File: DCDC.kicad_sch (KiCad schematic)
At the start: 18 parts, among them IC1 AZ1117CH-3.3TRG1

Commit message: コンデンサを追加
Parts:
- removed C10, C7: 10µF, Capacitor_SMD:C_0805_2012Metric_Pad1.18x1.45mm_HandSolder, symbol Device:C
- removed C10, C9: 47u, Capacitor_SMD:C_0805_2012Metric_Pad1.18x1.45mm_HandSolder, symbol Device:C
- removed C3: 0.1μF, Capacitor_SMD:C_0603_1608Metric_Pad1.08x0.95mm_HandSolder, symbol Device:C
- removed C4: 0.01μF, Capacitor_SMD:C_0603_1608Metric_Pad1.08x0.95mm_HandSolder, symbol Device:C
- removed C5, C6, C7, C8: 47u, Capacitor_SMD:C_1210_3225Metric_Pad1.33x2.70mm_HandSolder, symbol Device:C
- removed IC1: AZ1117CH-3.3TRG1, Library:SOT230P700X180-4N, symbol SamacSys_Parts:AZ1117CH-3.3TRG1
- removed L1: CDRH127_LDNP-560MC, Library:INDPM7066X300N, symbol CDRH127_LDNP-560MC:CDRH127_LDNP-560MC
- removed PS1: BP5293-50, Library:TO254P570X1700X1780-3P, symbol BP5293-50:BP5293-50
- removed R1, R2, R3: R, Resistor_SMD:R_0603_1608Metric_Pad0.98x0.95mm_HandSolder, symbol Device:R
- removed U1: ~, Package_SO:SOIC-8-1EP_3.9x4.9mm_P1.27mm_EP2.95x4.9mm_Mask2.71x3.4mm, symbol AP64502:AP64502
- removed VR1: 3362P-1-103LF, Library:3362P_1, symbol 3362P-1-103LF:3362P-1-103LF

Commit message: 電流センサー変更
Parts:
- added C10, C9: 47u, Capacitor_SMD:C_0805_2012Metric_Pad1.18x1.45mm_HandSolder, symbol Device:C
- added C3: 0.1μF, Capacitor_SMD:C_0603_1608Metric_Pad1.08x0.95mm_HandSolder, symbol Device:C
- added C4: 0.01μF, Capacitor_SMD:C_0603_1608Metric_Pad1.08x0.95mm_HandSolder, symbol Device:C
- added C45, C46: 10µF, Capacitor_SMD:C_0805_2012Metric_Pad1.18x1.45mm_HandSolder, symbol Device:C
- added C5, C6, C7, C8: 47u, Capacitor_SMD:C_1210_3225Metric_Pad1.33x2.70mm_HandSolder, symbol Device:C
- added IC11: AZ1117CH-3.3TRG1, Library:SOT230P700X180-4N, symbol SamacSys_Parts:AZ1117CH-3.3TRG1
- added L1: CDRH127_LDNP-560MC, Library:INDPM7066X300N, symbol CDRH127_LDNP-560MC:CDRH127_LDNP-560MC
- added PS2: BP5293-50, Library:TO254P570X1700X1780-3P, symbol BP5293-50:BP5293-50
- added R1 (x2): 100kΩ, Resistor_SMD:R_0603_1608Metric_Pad0.98x0.95mm_HandSolder, symbol Device:R
- added R2, R3: R, Resistor_SMD:R_0603_1608Metric_Pad0.98x0.95mm_HandSolder, symbol Device:R
- added U1: ~, Package_SO:SOIC-8-1EP_3.9x4.9mm_P1.27mm_EP2.95x4.9mm_Mask2.71x3.4mm, symbol AP64502:AP64502
- added VR1: 3362P-1-103LF, Library:3362P_1, symbol 3362P-1-103LF:3362P-1-103LF
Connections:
- new net: C3.2, L1.1, U1.8 (SW)
- new net: R1.1, U1.4 (RT/CLK)
- new net: R1.1, R1.2
- new net: R2.1, VR1.2 (WIPER)
- new net: R2.2, R3.1, U1.5 (FB)
- new net: C4.1, U1.6 (SS)
- new net: C3.1, U1.1 (BST)
- new net +5V: C45.1, IC11.3 (INPUT), PS2.3 (VOUT)
- new net 3.3V: C46.1, IC11.2 (OUTPUT), IC11.4 (VOUT)
- new net GND: C10.2, C4.2, C45.2, C46.2, C5.2, C6.2, C7.2, C8.2, C9.2, IC11.1 (ADJ/GND), PS2.2 (GND), R1.2, R3.2, U1.7 (GND), U1.9 (GND)
- new net VIN: C10.1, C9.1, PS2.1 (VIN), U1.2 (VIN), U1.3 (EN)
- new net VOUT: C5.1, C6.1, C7.1, C8.1, L1.2, VR1.3 (CW)

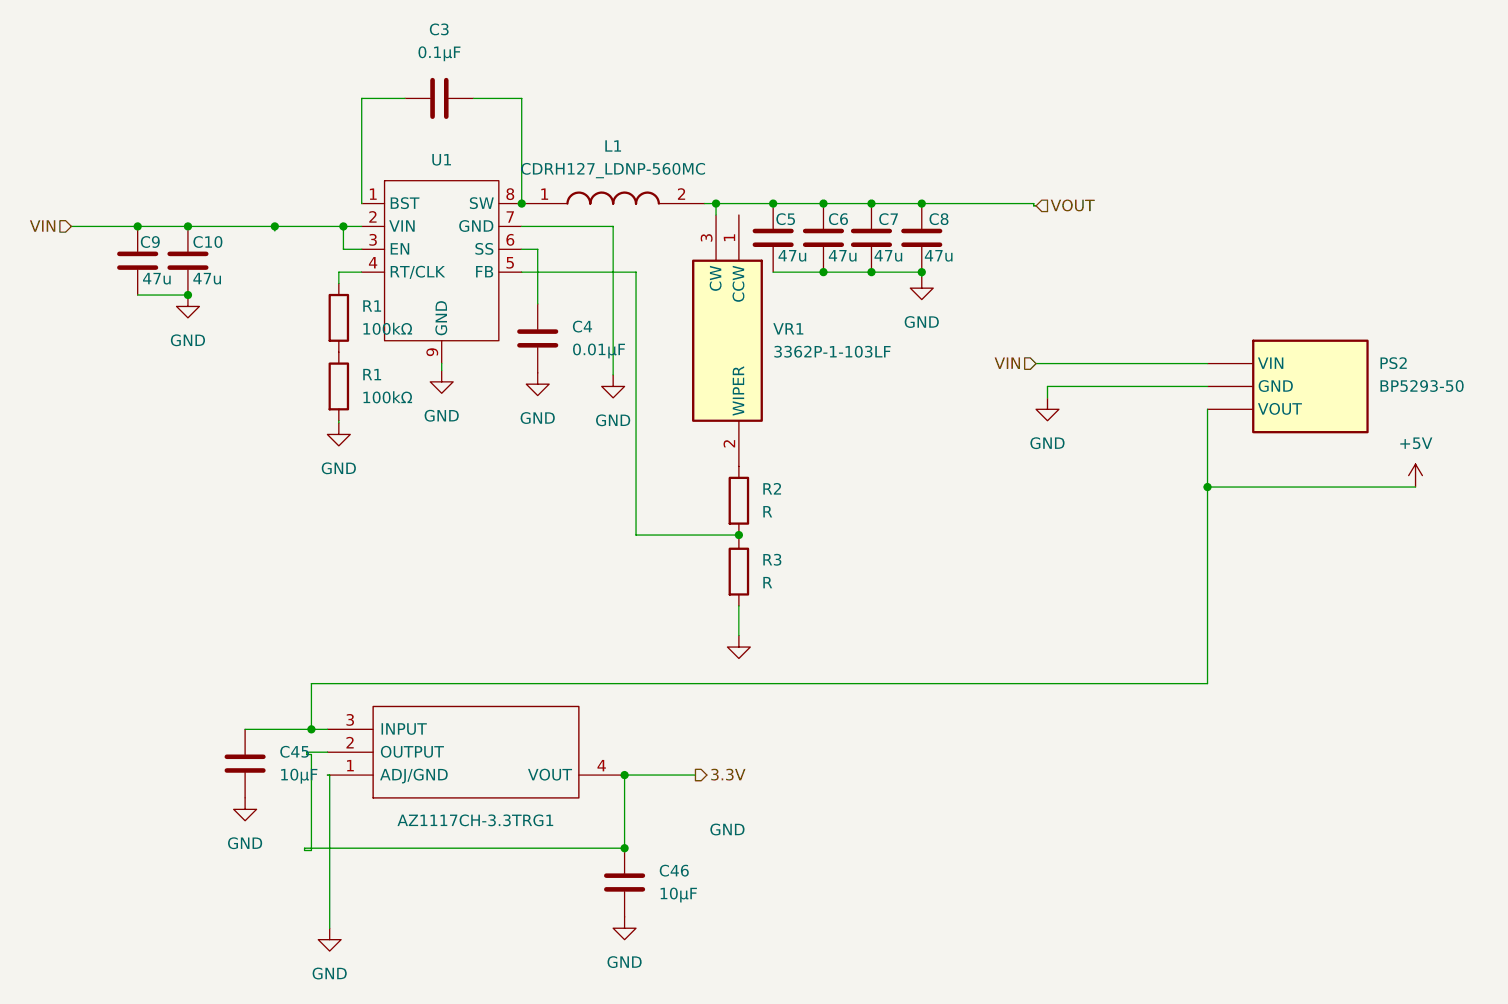
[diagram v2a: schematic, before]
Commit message: ESP32バージョン
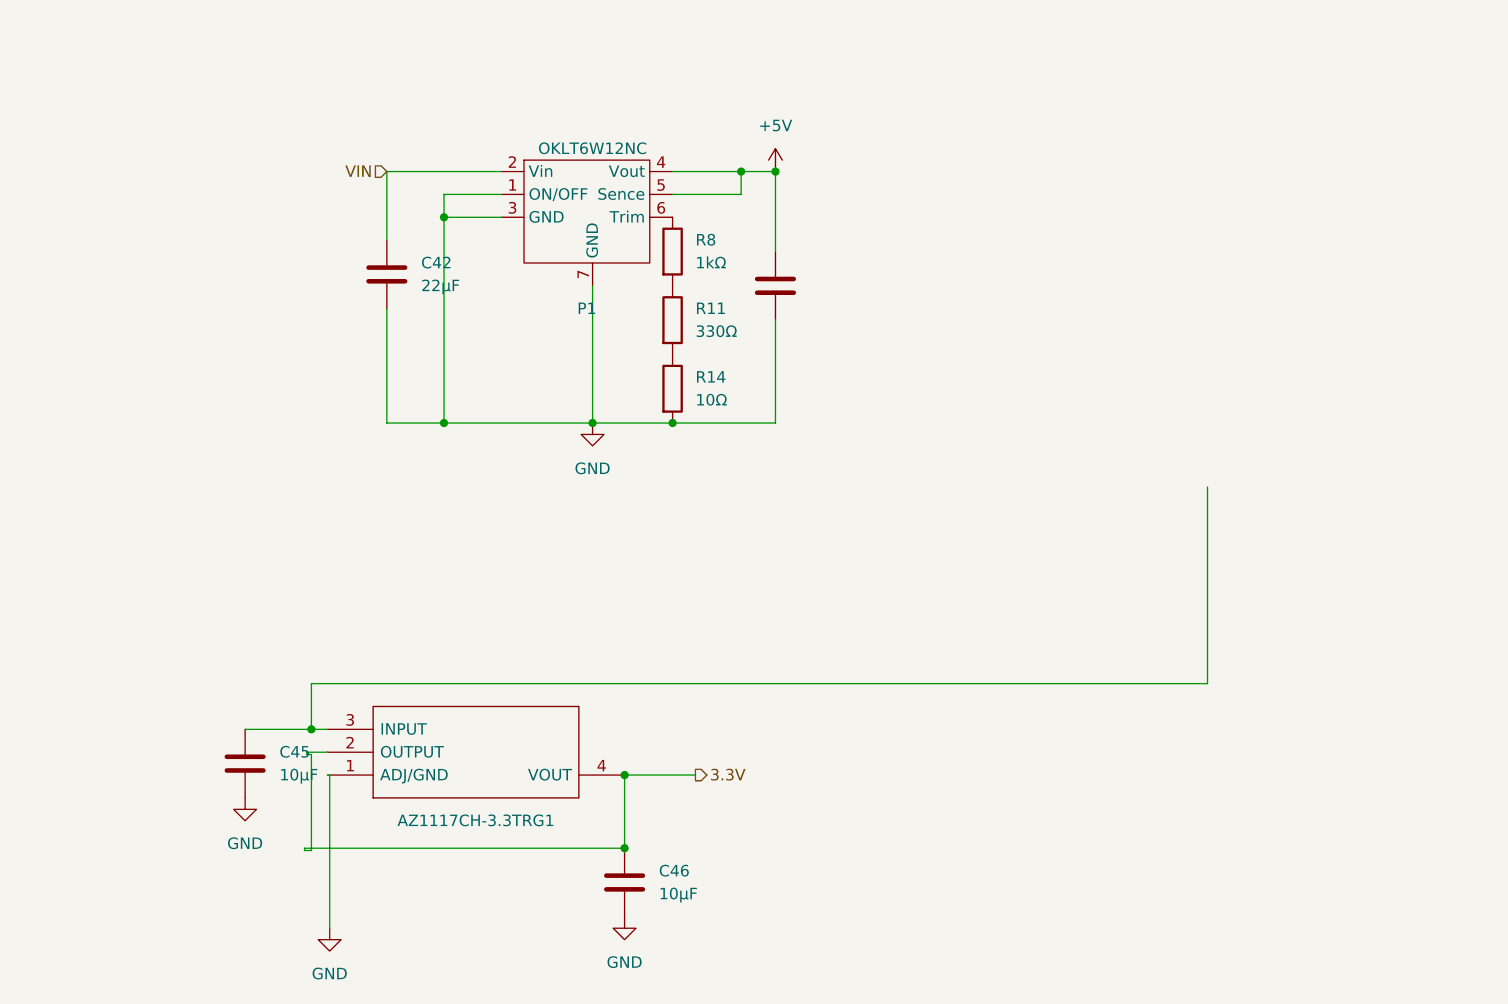
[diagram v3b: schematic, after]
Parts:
- removed C10, C9: 47u, Capacitor_SMD:C_0805_2012Metric_Pad1.18x1.45mm_HandSolder, symbol Device:C
- removed C3: 0.1μF, Capacitor_SMD:C_0603_1608Metric_Pad1.08x0.95mm_HandSolder, symbol Device:C
- removed C4: 0.01μF, Capacitor_SMD:C_0603_1608Metric_Pad1.08x0.95mm_HandSolder, symbol Device:C
- removed C5, C6, C7, C8: 47u, Capacitor_SMD:C_1210_3225Metric_Pad1.33x2.70mm_HandSolder, symbol Device:C
- removed L1: CDRH127_LDNP-560MC, Library:INDPM7066X300N, symbol CDRH127_LDNP-560MC:CDRH127_LDNP-560MC
- removed PS2: BP5293-50, Library:TO254P570X1700X1780-3P, symbol BP5293-50:BP5293-50
- removed R1 (x2): 100kΩ, Resistor_SMD:R_0603_1608Metric_Pad0.98x0.95mm_HandSolder, symbol Device:R
- removed R2, R3: R, Resistor_SMD:R_0603_1608Metric_Pad0.98x0.95mm_HandSolder, symbol Device:R
- removed U1: ~, Package_SO:SOIC-8-1EP_3.9x4.9mm_P1.27mm_EP2.95x4.9mm_Mask2.71x3.4mm, symbol AP64502:AP64502
- removed VR1: 3362P-1-103LF, Library:3362P_1, symbol 3362P-1-103LF:3362P-1-103LF
- added C42: 22μF, Capacitor_SMD:C_0805_2012Metric_Pad1.18x1.45mm_HandSolder, symbol Device:C
- added C44: 10μF, Capacitor_SMD:C_0805_2012Metric_Pad1.18x1.45mm_HandSolder, symbol Device:C
- added P1: OKLT6W12NC, Library:OKLT6W12NC, symbol OKL_sym:OKL_T6_W12
- added R11: 330Ω, Resistor_SMD:R_0805_2012Metric_Pad1.20x1.40mm_HandSolder, symbol Device:R
- added R14: 10Ω, Resistor_SMD:R_0805_2012Metric_Pad1.20x1.40mm_HandSolder, symbol Device:R
- added R8: 1kΩ, Resistor_SMD:R_0805_2012Metric_Pad1.20x1.40mm_HandSolder, symbol Device:R
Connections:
- net +5V: now also C44.1, P1.4 (Vout), P1.5 (Sence); no longer C45.1, IC11.3 (INPUT)
- net GND: now also C42.2, C44.2, P1.1 (ON/OFF), P1.3 (GND), P1.7 (GND), R14.2
- net VIN: now also C42.1, P1.2 (Vin)
- new net: R11.1, R8.2
- new net: R11.2, R14.1
- new net: C45.1, IC11.3 (INPUT)
- new net: P1.6 (Trim), R8.1
